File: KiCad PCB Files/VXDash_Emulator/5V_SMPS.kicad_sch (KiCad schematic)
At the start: 13 parts, among them IC4 AP62200

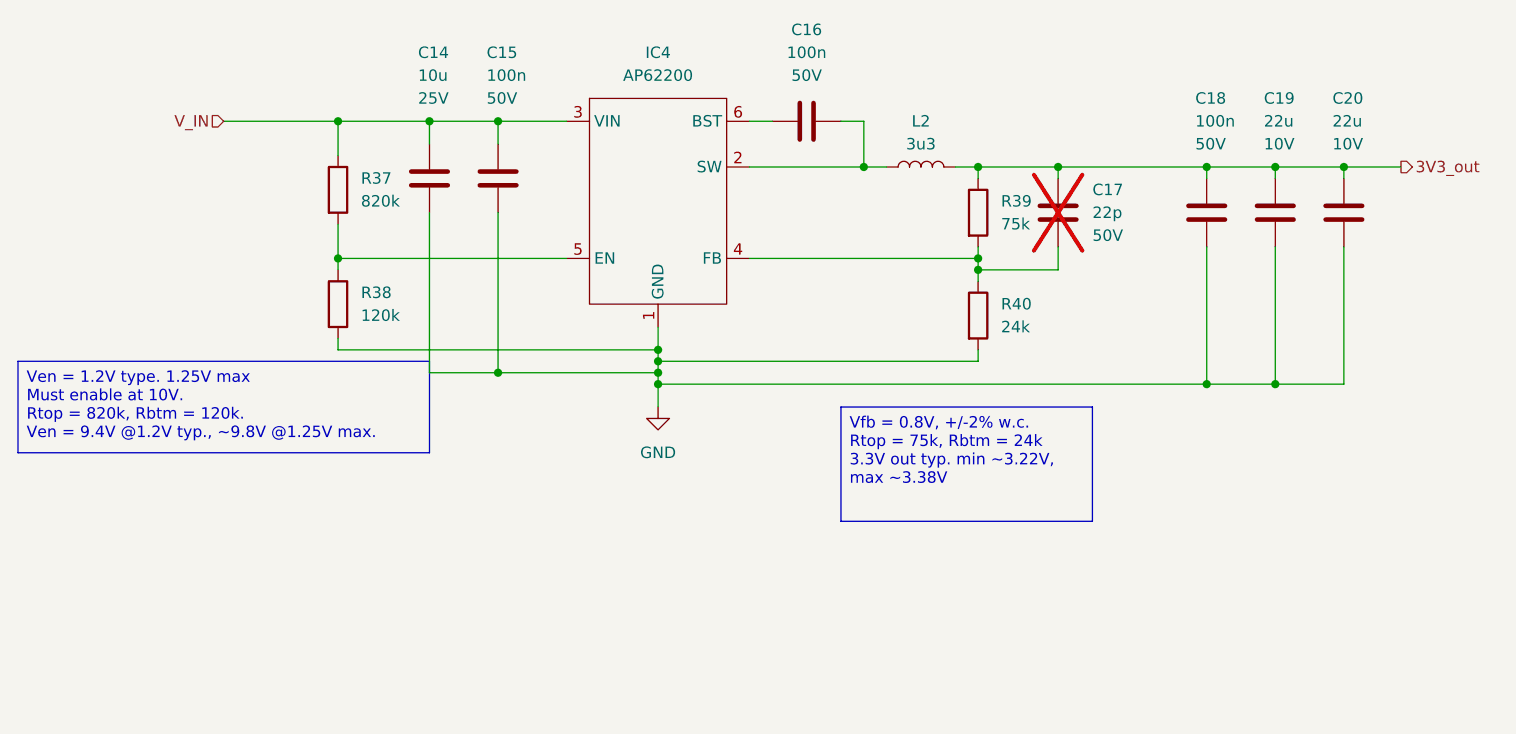
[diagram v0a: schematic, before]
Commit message: More changes (Primarily Remote ECU)
- Emulator board project to a functional skeleton
- Connectors board with ignition routing on CAN pin 4 to have switched signal available in the harness.
- Remote ECU : added 12V reduced protection circuit (to be reviewed)
- Remote ECU : Removed integrated CAN termination (should be on harness)
- Remote ECU : added CAN passthrough
- Remote ECU : added MCPWM channels
- Remote ECU : Added some opto inputs
- Remote ECU : Added internal USB C (overkill ?)
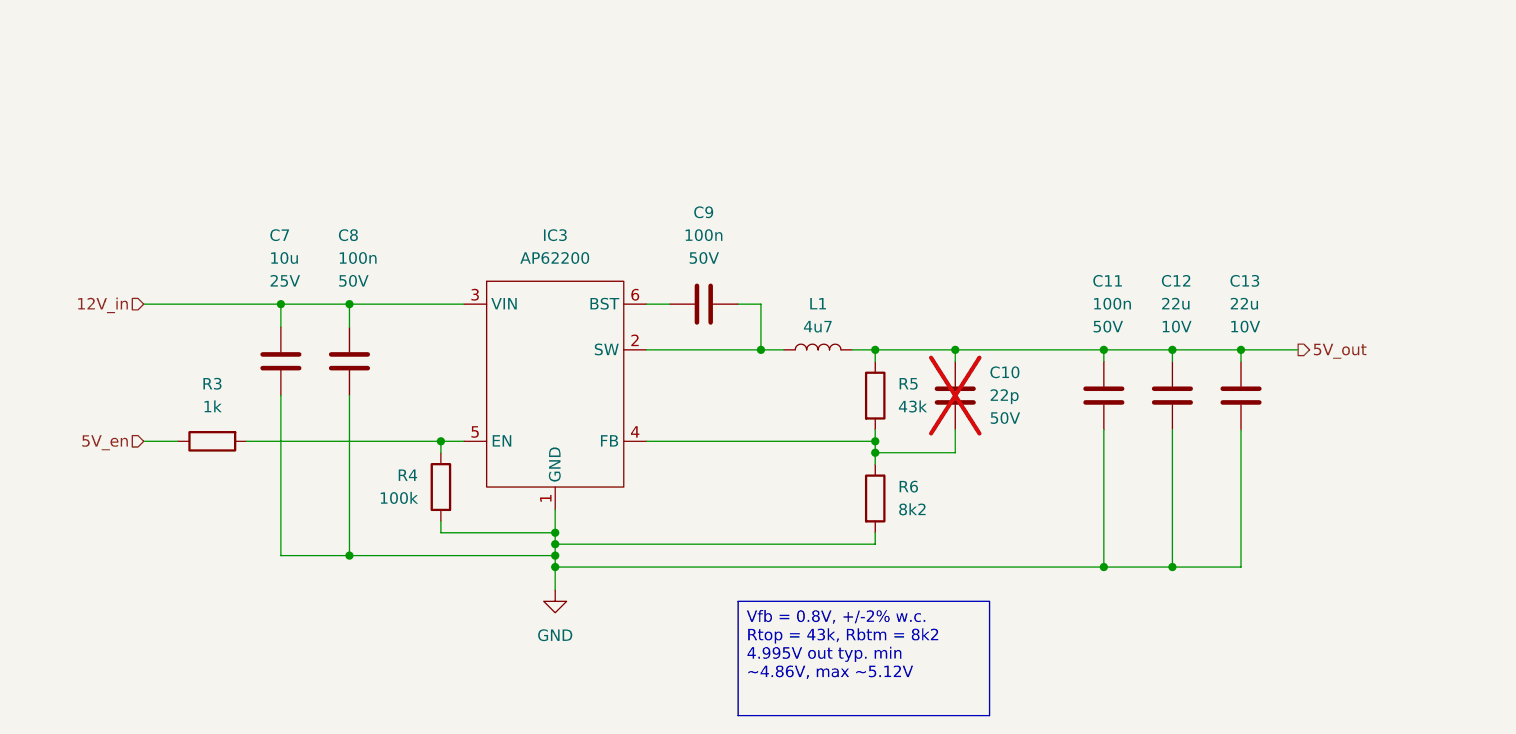
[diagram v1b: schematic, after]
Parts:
- removed C14: 10u, Capacitor_SMD:C_1206_3216Metric_Pad1.33x1.80mm_HandSolder, symbol VXDash_passives:Cap_MLCC
- removed C15, C16, C18: 100n, symbol VXDash_passives:Cap_MLCC
- removed C17: 22p, Capacitor_SMD:C_0402_1005Metric_Pad0.74x0.62mm_HandSolder, symbol VXDash_passives:Cap_MLCC
- removed C19, C20: 22u, Capacitor_SMD:C_1206_3216Metric_Pad1.33x1.80mm_HandSolder, symbol VXDash_passives:Cap_MLCC
- removed IC4: AP62200, Package_TO_SOT_SMD:TSOT-23-6_HandSoldering, symbol VXDash_regulators:AP62200
- removed L2: 3u3, Inductor_SMD:L_Taiyo-Yuden_NR-50xx_HandSoldering, symbol VXDash_passives:Ind
- removed R37: 820k, Resistor_SMD:R_0603_1608Metric_Pad0.98x0.95mm_HandSolder, symbol VXDash_passives:Res
- removed R38: 120k, Resistor_SMD:R_0603_1608Metric_Pad0.98x0.95mm_HandSolder, symbol VXDash_passives:Res
- removed R39: 75k, Resistor_SMD:R_0603_1608Metric_Pad0.98x0.95mm_HandSolder, symbol VXDash_passives:Res
- removed R40: 24k, Resistor_SMD:R_0603_1608Metric_Pad0.98x0.95mm_HandSolder, symbol VXDash_passives:Res
- added C10: 22p, Capacitor_SMD:C_0402_1005Metric_Pad0.74x0.62mm_HandSolder, symbol VXDash_passives:Cap_MLCC
- added C11, C8, C9: 100n, symbol VXDash_passives:Cap_MLCC
- added C12, C13: 22u, Capacitor_SMD:C_1206_3216Metric_Pad1.33x1.80mm_HandSolder, symbol VXDash_passives:Cap_MLCC
- added C7: 10u, Capacitor_SMD:C_1206_3216Metric_Pad1.33x1.80mm_HandSolder, symbol VXDash_passives:Cap_MLCC
- added IC3: AP62200, Package_TO_SOT_SMD:TSOT-23-6_HandSoldering, symbol VXDash_regulators:AP62200
- added L1: 4u7, VXDash_inductors:Ind_5050, symbol VXDash_passives:Ind
- added R3: 1k, Resistor_SMD:R_0603_1608Metric_Pad0.98x0.95mm_HandSolder, symbol VXDash_passives:Res
- added R4: 100k, Resistor_SMD:R_0603_1608Metric_Pad0.98x0.95mm_HandSolder, symbol VXDash_passives:Res
- added R5: 43k, Resistor_SMD:R_0603_1608Metric_Pad0.98x0.95mm_HandSolder, symbol VXDash_passives:Res
- added R6: 8k2, Resistor_SMD:R_0603_1608Metric_Pad0.98x0.95mm_HandSolder, symbol VXDash_passives:Res
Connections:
- net GND: now also C11.1, C12.2, C13.2, C7.1, C8.1, IC3.1 (GND), R4.2, R6.2
- new net: C10.2, IC3.4 (FB), R5.2, R6.1
- new net: C9.1, IC3.2 (SW), L1.1
- new net: IC3.5 (EN), R3.2, R4.1
- new net: C9.2, IC3.6 (BST)
- new net 12V_in: C7.2, C8.2, IC3.3 (VIN)
- new net 5V_en: R3.1
- new net 5V_out: C10.1, C11.2, C12.1, C13.1, L1.2, R5.1
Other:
- company: (none) -> Alex Miller & Martin Roger
- title: VXDash RemoteECU -> Main architecture

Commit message: ERC corrections, idiot lights
- VXDash : added idiot lights (also to emulator board)
- VXDash : corrected some ERC violations
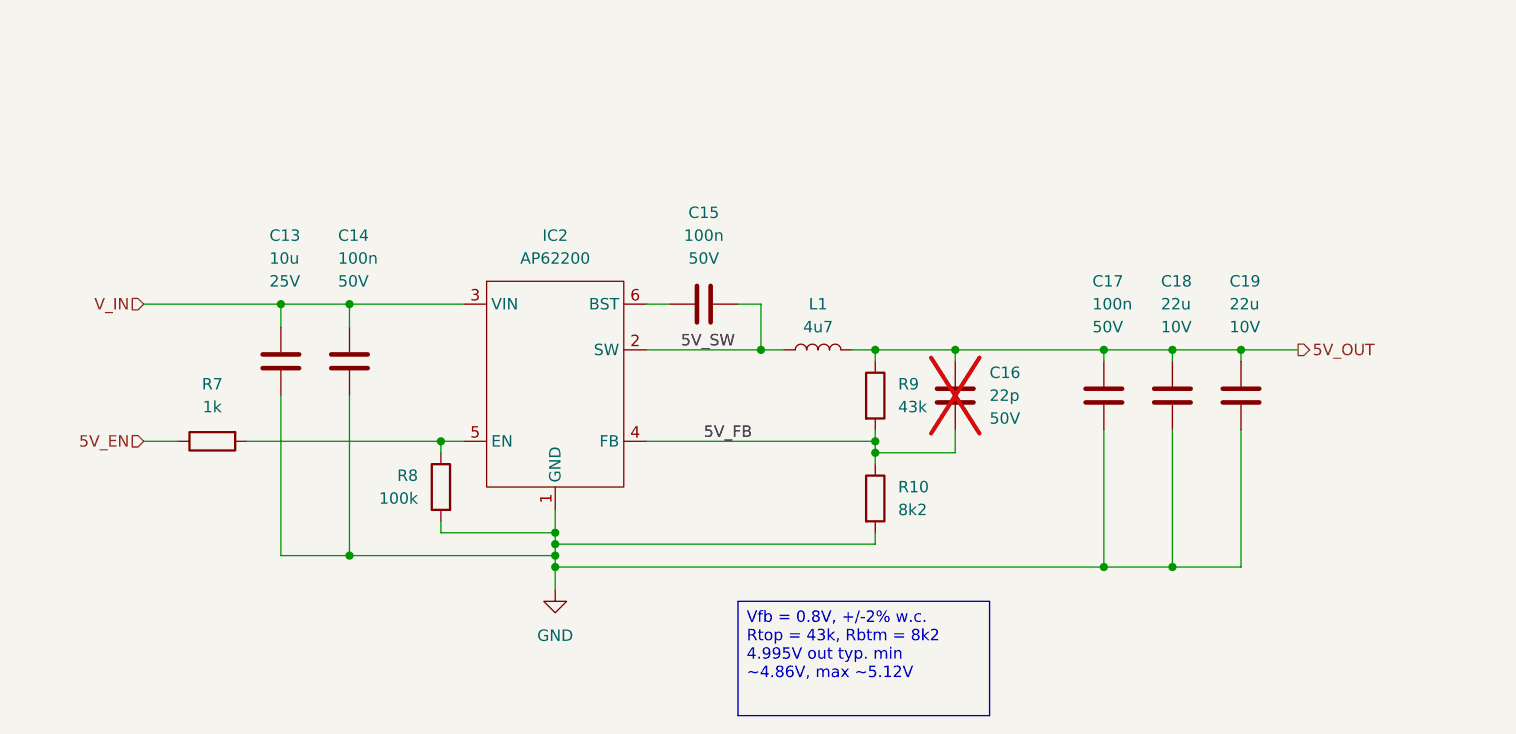
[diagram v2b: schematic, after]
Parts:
- C14: renamed from C8; footprint (none) -> Capacitor_SMD:C_0603_1608Metric_Pad1.08x0.95mm_HandSolder
- C15: renamed from C9; footprint (none) -> Capacitor_SMD:C_0603_1608Metric_Pad1.08x0.95mm_HandSolder
- C17: renamed from C11; footprint (none) -> Capacitor_SMD:C_0603_1608Metric_Pad1.08x0.95mm_HandSolder
- renumbered C7 to C13, C10 to C16, C12 to C18, C13 to C19, IC3 to IC2, R6 to R10, R3 to R7, R4 to R8, R5 to R9
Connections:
- net 5V_FB: now reaches C16.2, IC2.4 (FB), R10.1, R9.2
- net 5V_SW: now reaches C15.1, IC2.2 (SW), L1.1
- net 12V_in renamed V_IN
- net 5V_en renamed 5V_EN
- net 5V_out renamed 5V_OUT
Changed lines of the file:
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@@
 		(title "Main architecture")
 		(date "2025-08-10")
-		(rev "0.0")
+		(rev "1.4")
 		(company "Alex Miller & Martin Roger")
 		(comment 1 "https://github.com/martinroger/VXDash")
@@
 		)
 	)
-	(hierarchical_label "12V_in"
+	(label "5V_SW"
+		(at 127 81.28 0)
+		(effects
+			(font
+				(size 1.27 1.27)
+			)
+			(justify left bottom)
+		)
+	)
+	(label "5V_FB"
+		(at 129.54 91.44 0)
+		(effects
+			(font
+				(size 1.27 1.27)
+			)
+			(justify left bottom)
+		)
+	)
+	(hierarchical_label "V_IN"
 		(shape input)
 		(at 67.31 76.2 180)
@@
 		)
 	)
-	(hierarchical_label "5V_out"
+	(hierarchical_label "5V_OUT"
 		(shape output)
 		(at 195.58 81.28 0)
@@
 		)
 	)
-	(hierarchical_label "5V_en"
+	(hierarchical_label "5V_EN"
 		(shape input)
 		(at 67.31 91.44 180)
@@
 		(dnp no)
 		(fields_autoplaced yes)
-		(property "Reference" "#PWR012"
+		(property "Reference" "#PWR022"
 			(at 113.03 114.3 0)
 			(effects
@@
 			(project "VXDash"
 				(path "/f2858fc4-50de-4ff0-a01c-5b985ee14aef/e4c69d46-7a64-435d-9e3a-d73acbe7ec2b"
-					(reference "#PWR012")
+					(reference "#PWR022")
 					(unit 1)
 				)
@@
 		(dnp yes)
 		(fields_autoplaced yes)
-		(property "Reference" "C10"
+		(property "Reference" "C16"
 			(at 161.29 83.8199 0)
 			(effects
@@
 		)
 		(property "MFT_PN" ""
+			(at 157.48 86.36 0)
+			(effects
+				(font
+					(size 1.27 1.27)
+				)
+				(hide yes)
+			)
+		)
+		(property "Tolerance" ""
 			(at 157.48 86.36 0)
 			(effects
@@
 			(project "VXDash"
 				(path "/f2858fc4-50de-4ff0-a01c-5b985ee14aef/e4c69d46-7a64-435d-9e3a-d73acbe7ec2b"
-					(reference "C10")
+					(reference "C16")
 					(unit 1)
 				)
@@
 		(on_board yes)
 		(dnp no)
-		(property "Reference" "C8"
+		(property "Reference" "C14"
 			(at 88.9 68.58 0)
 			(effects
@@
 			)
 		)
-		(property "Footprint" ""
+		(property "Footprint" "Capacitor_SMD:C_0603_1608Metric_Pad1.08x0.95mm_HandSolder"
 			(at 91.1352 78.74 0)
 			(effects
@@
 				)
 				(justify left)
+			)
+		)
+		(property "Tolerance" ""
+			(at 90.17 82.55 0)
+			(effects
+				(font
+					(size 1.27 1.27)
+				)
+				(hide yes)
 			)
 		)
@@
 			(project "VXDash"
 				(path "/f2858fc4-50de-4ff0-a01c-5b985ee14aef/e4c69d46-7a64-435d-9e3a-d73acbe7ec2b"
-					(reference "C8")
+					(reference "C14")
 					(unit 1)
 				)
@@
 		(on_board yes)
 		(dnp no)
-		(property "Reference" "C13"
+		(property "Reference" "C19"
 			(at 187.96 73.66 0)
 			(effects
@@
 		)
 		(property "MFT_PN" ""
+			(at 189.23 86.36 0)
+			(effects
+				(font
+					(size 1.27 1.27)
+				)
+				(hide yes)
+			)
+		)
+		(property "Tolerance" ""
 			(at 189.23 86.36 0)
 			(effects
@@
 			(project "VXDash"
 				(path "/f2858fc4-50de-4ff0-a01c-5b985ee14aef/e4c69d46-7a64-435d-9e3a-d73acbe7ec2b"
-					(reference "C13")
+					(reference "C19")
 					(unit 1)
 				)
@@
 		(on_board yes)
 		(dnp no)
-		(property "Reference" "C12"
+		(property "Reference" "C18"
 			(at 180.34 73.66 0)
 			(effects
@@
 		)
 		(property "MFT_PN" ""
+			(at 181.61 86.36 0)
+			(effects
+				(font
+					(size 1.27 1.27)
+				)
+				(hide yes)
+			)
+		)
+		(property "Tolerance" ""
 			(at 181.61 86.36 0)
 			(effects
@@
 			(project "VXDash"
 				(path "/f2858fc4-50de-4ff0-a01c-5b985ee14aef/e4c69d46-7a64-435d-9e3a-d73acbe7ec2b"
-					(reference "C12")
+					(reference "C18")
 					(unit 1)
 				)
@@
 		(dnp no)
 		(fields_autoplaced yes)
-		(property "Reference" "IC3"
+		(property "Reference" "IC2"
 			(at 113.03 68.58 0)
 			(effects
@@
 		(property "MFT_PN" "AP62200WU-7"
 			(at 113.03 58.42 0)
+			(effects
+				(font
+					(size 1.27 1.27)
+				)
+				(hide yes)
+			)
+		)
+		(property "Tolerance" ""
+			(at 113.03 73.66 0)
 			(effects
 				(font
@@
 			(project "VXDash"
 				(path "/f2858fc4-50de-4ff0-a01c-5b985ee14aef/e4c69d46-7a64-435d-9e3a-d73acbe7ec2b"
-					(reference "IC3")
+					(reference "IC2")
 					(unit 1)
 				)
@@
 		(dnp no)
 		(fields_autoplaced yes)
-		(property "Reference" "R3"
+		(property "Reference" "R7"
 			(at 74.93 85.09 90)
 			(effects
@@
 		(property "MFT_PN" ""
 			(at 74.93 91.44 0)
+			(effects
+				(font
+					(size 1.27 1.27)
+				)
+				(hide yes)
+			)
+		)
+		(property "Tolerance" ""
+			(at 74.93 91.44 90)
 			(effects
 				(font
@@
 			(project "VXDash"
 				(path "/f2858fc4-50de-4ff0-a01c-5b985ee14aef/e4c69d46-7a64-435d-9e3a-d73acbe7ec2b"
-					(reference "R3")
+					(reference "R7")
 					(unit 1)
 				)
@@
 			)
 		)
+		(property "Tolerance" ""
+			(at 142.24 81.28 0)
+			(effects
+				(font
+					(size 1.27 1.27)
+				)
+				(hide yes)
+			)
+		)
 		(pin "2"
 		)
@@
 		(dnp no)
 		(fields_autoplaced yes)
-		(property "Reference" "C9"
+		(property "Reference" "C15"
 			(at 129.54 66.04 90)
 			(effects
@@
 			)
 		)
-		(property "Footprint" ""
+		(property "Footprint" "Capacitor_SMD:C_0603_1608Metric_Pad1.08x0.95mm_HandSolder"
 			(at 125.73 75.2348 0)
 			(effects
@@
 					(size 1.27 1.27)
 				)
+			)
+		)
+		(property "Tolerance" ""
+			(at 129.54 76.2 90)
+			(effects
+				(font
+					(size 1.27 1.27)
+				)
+				(hide yes)
 			)
 		)
@@
 			(project "VXDash"
 				(path "/f2858fc4-50de-4ff0-a01c-5b985ee14aef/e4c69d46-7a64-435d-9e3a-d73acbe7ec2b"
-					(reference "C9")
+					(reference "C15")
 					(unit 1)
 				)
@@
 		(on_board yes)
 		(dnp no)
-		(property "Reference" "C11"
+		(property "Reference" "C17"
 			(at 172.72 73.66 0)
 			(effects
@@
 			)
 		)
-		(property "Footprint" ""
+		(property "Footprint" "Capacitor_SMD:C_0603_1608Metric_Pad1.08x0.95mm_HandSolder"
 			(at 174.9552 82.55 0)
 			(effects
@@
 				)
 				(justify left)
+			)
+		)
+		(property "Tolerance" ""
+			(at 173.99 86.36 0)
+			(effects
+				(font
+					(size 1.27 1.27)
+				)
+				(hide yes)
 			)
 		)
@@
 			(project "VXDash"
 				(path "/f2858fc4-50de-4ff0-a01c-5b985ee14aef/e4c69d46-7a64-435d-9e3a-d73acbe7ec2b"
-					(reference "C11")
+					(reference "C17")
 					(unit 1)
 				)
@@
 		(dnp no)
 		(fields_autoplaced yes)
-		(property "Reference" "R6"
+		(property "Reference" "R10"
 			(at 151.13 96.5199 0)
 			(effects
@@
 		)
 		(property "MFT_PN" ""
+			(at 148.59 97.79 0)
+			(effects
+				(font
+					(size 1.27 1.27)
+				)
+				(hide yes)
+			)
+		)
+		(property "Tolerance" ""
 			(at 148.59 97.79 0)
 			(effects
@@
 			(project "VXDash"
 				(path "/f2858fc4-50de-4ff0-a01c-5b985ee14aef/e4c69d46-7a64-435d-9e3a-d73acbe7ec2b"
-					(reference "R6")
+					(reference "R10")
 					(unit 1)
 				)
@@
 		(on_board yes)
 		(dnp no)
-		(property "Reference" "C7"
+		(property "Reference" "C13"
 			(at 81.28 68.58 0)
 			(effects
@@
 				)
 				(justify left)
+			)
+		)
+		(property "Tolerance" ""
+			(at 82.55 82.55 0)
+			(effects
+				(font
+					(size 1.27 1.27)
+				)
+				(hide yes)
 			)
 		)
@@
 			(project "VXDash"
 				(path "/f2858fc4-50de-4ff0-a01c-5b985ee14aef/e4c69d46-7a64-435d-9e3a-d73acbe7ec2b"
-					(reference "C7")
+					(reference "C13")
 					(unit 1)
 				)
@@
 		(dnp no)
 		(fields_autoplaced yes)
-		(property "Reference" "R4"
+		(property "Reference" "R8"
 			(at 97.79 95.2499 0)
 			(effects
@@
 		)
 		(property "MFT_PN" ""
+			(at 100.33 96.52 0)
+			(effects
+				(font
+					(size 1.27 1.27)
+				)
+				(hide yes)
+			)
+		)
+		(property "Tolerance" ""
 			(at 100.33 96.52 0)
 			(effects
@@
 			(project "VXDash"
 				(path "/f2858fc4-50de-4ff0-a01c-5b985ee14aef/e4c69d46-7a64-435d-9e3a-d73acbe7ec2b"
-					(reference "R4")
+					(reference "R8")
 					(unit 1)
 				)
@@
 		(dnp no)
 		(fields_autoplaced yes)
-		(property "Reference" "R5"
+		(property "Reference" "R9"
 			(at 151.13 85.0899 0)
 			(effects
@@
 		)
 		(property "MFT_PN" ""
+			(at 148.59 86.36 0)
+			(effects
+				(font
+					(size 1.27 1.27)
+				)
+				(hide yes)
+			)
+		)
+		(property "Tolerance" ""
 			(at 148.59 86.36 0)
 			(effects
@@
 			(project "VXDash"
 				(path "/f2858fc4-50de-4ff0-a01c-5b985ee14aef/e4c69d46-7a64-435d-9e3a-d73acbe7ec2b"
-					(reference "R5")
+					(reference "R9")
 					(unit 1)
 				)
